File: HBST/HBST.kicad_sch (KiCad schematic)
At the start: 14 parts, among them J1 Conn_01x06_Pin, J3 Conn_01x04_Pin, J4 Conn_01x13_Pin, J5 Conn_01x09_Pin

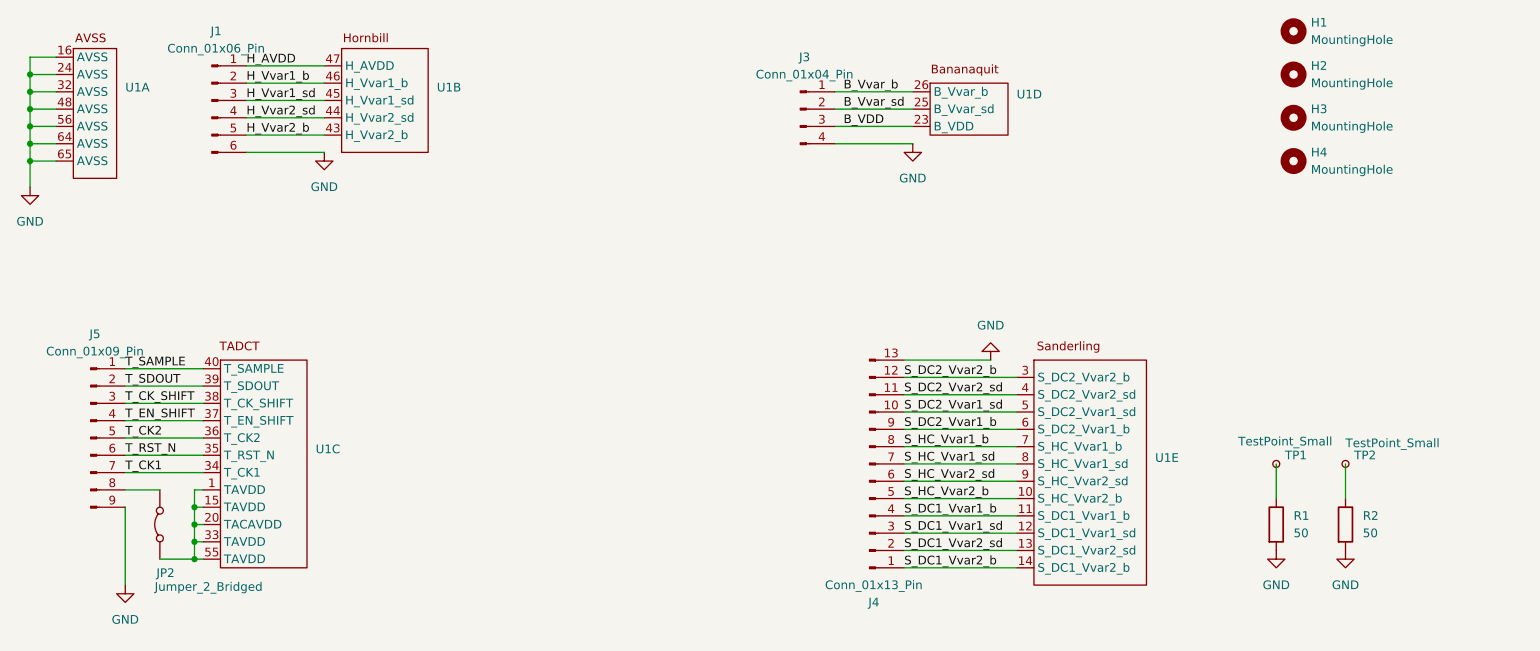
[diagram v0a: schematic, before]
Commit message: updated design
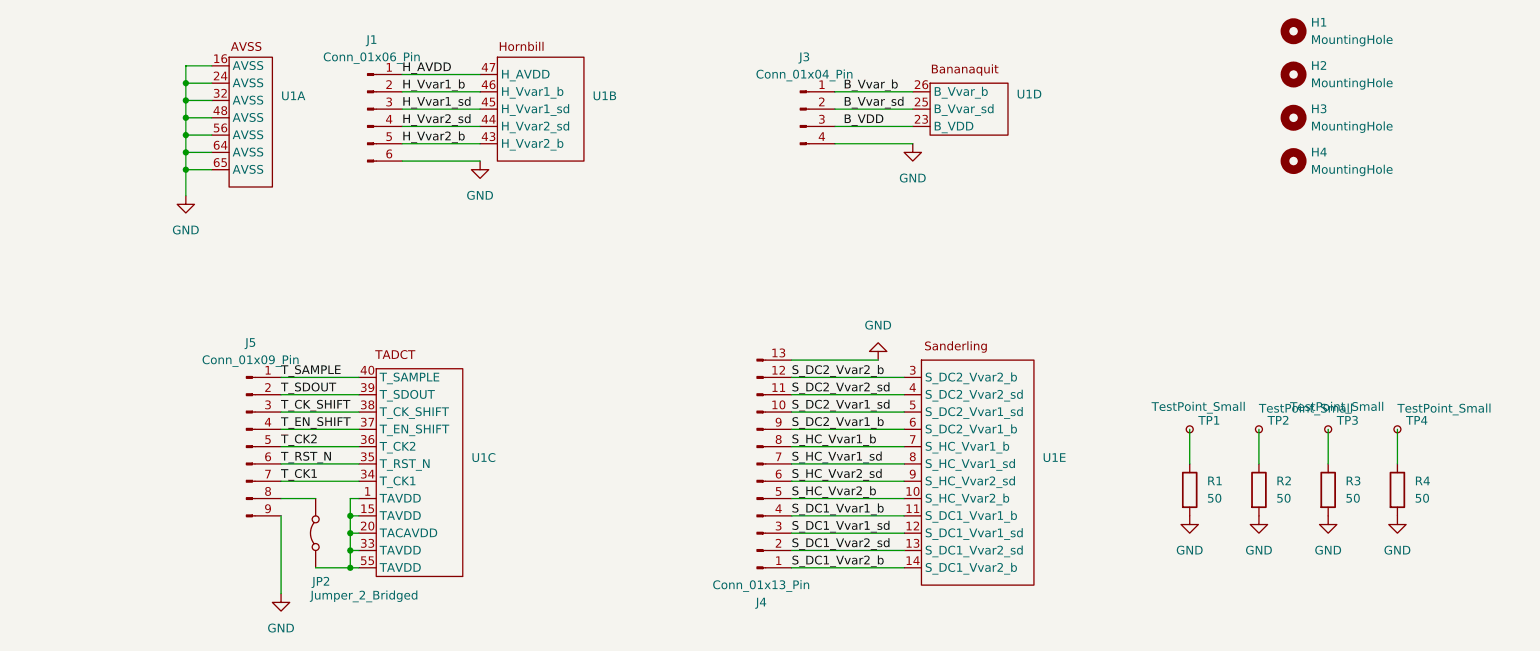
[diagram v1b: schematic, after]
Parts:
- added R3, R4: 50, Resistor_SMD:R_0805_2012Metric_Pad1.20x1.40mm_HandSolder, symbol Device:R
- added TP3, TP4: TestPoint_Small, TestPoint:TestPoint_Pad_D1.0mm, symbol Connector:TestPoint_Small
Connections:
- net GND: now also R3.2, R4.2
- new net: R3.1, TP3.1
- new net: R4.1, TP4.1
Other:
- moved on the sheet: J1, J4, J5, JP2, R1, R2, TP1, TP2, U1A, U1B, U1C, U1E
